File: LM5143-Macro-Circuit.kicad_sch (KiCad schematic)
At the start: 54 parts, among them J4 Conn_01x01_Socket, U1 LM5145, U2 NTMFS4D0N08XT1G, U3 NTMFS4D0N08XT1G, U4 NTMFS4D0N08XT1G, U5 NTMFS4D0N08XT1G

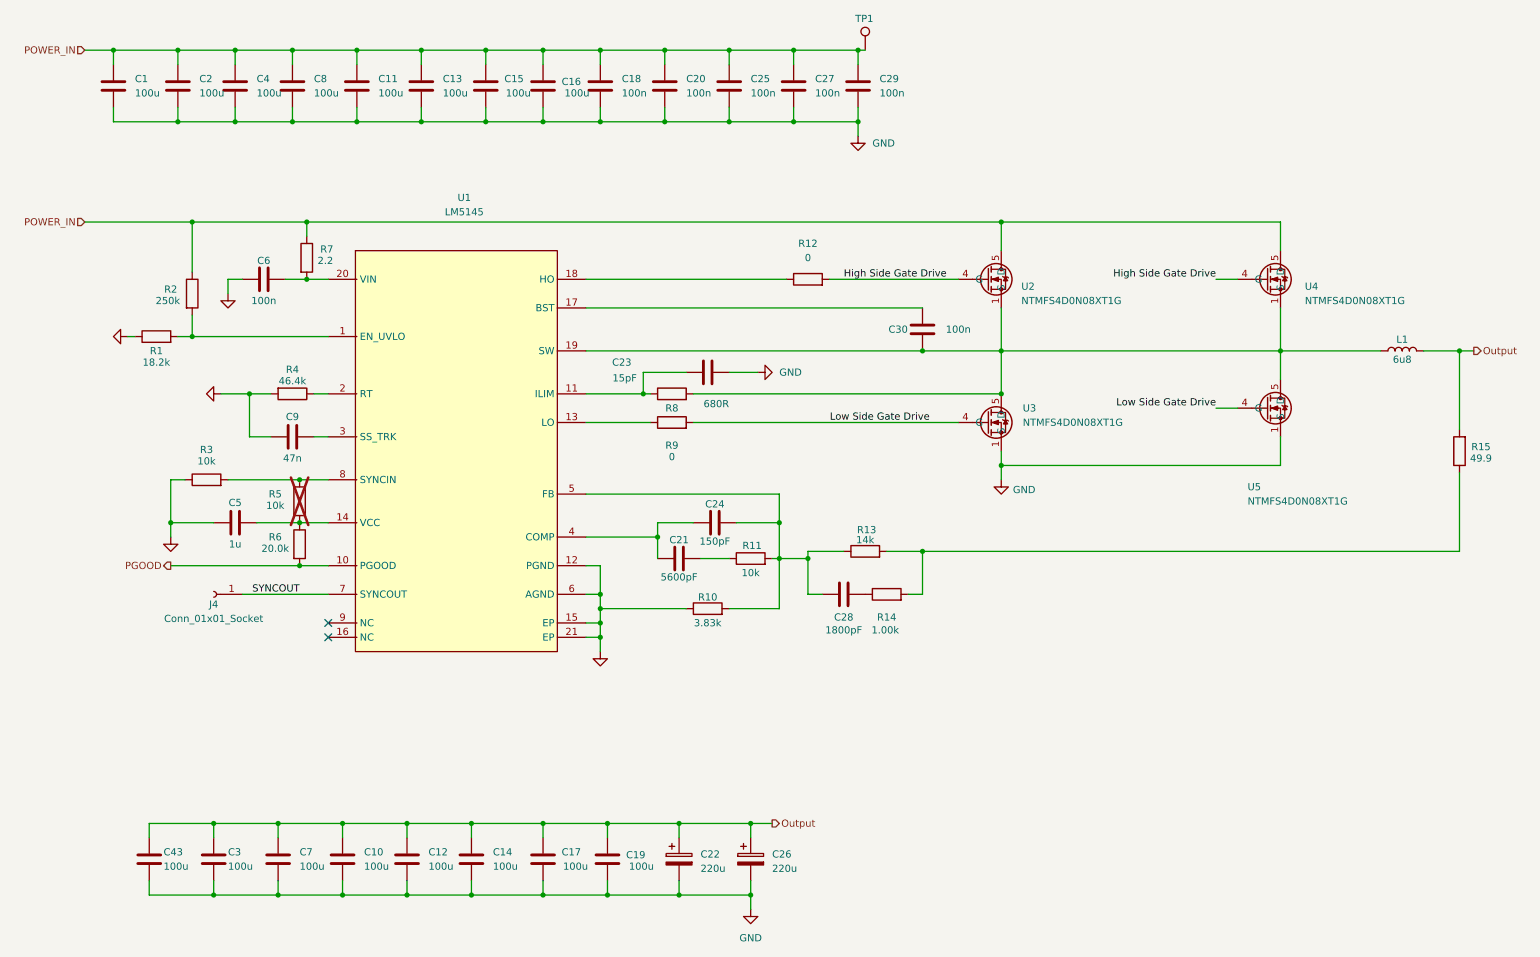
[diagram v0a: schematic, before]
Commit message: A
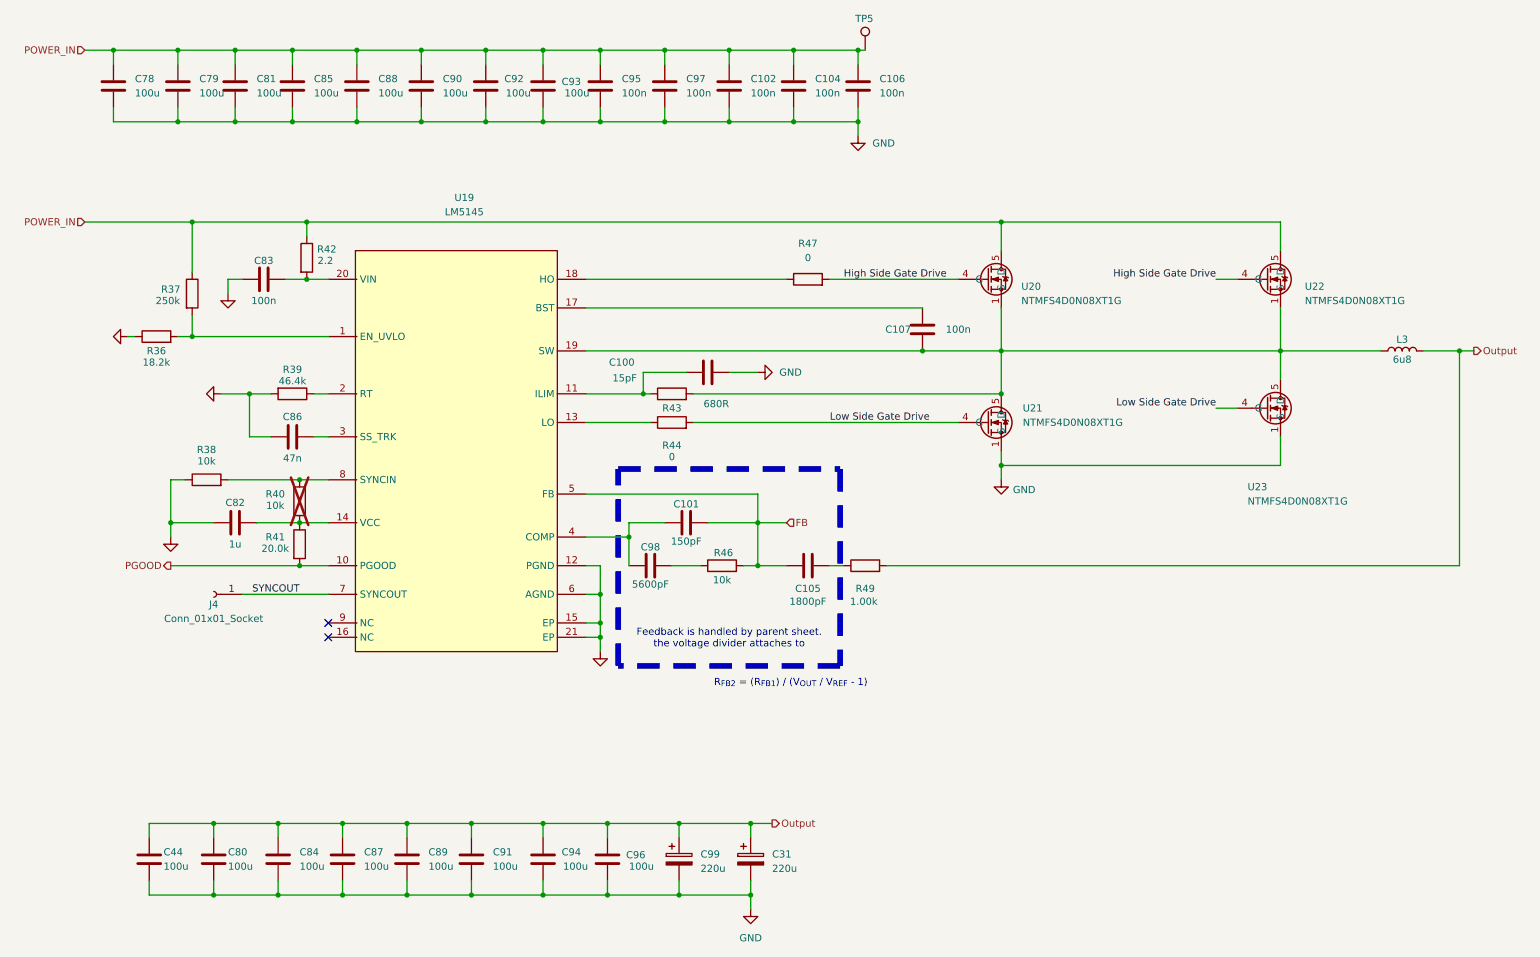
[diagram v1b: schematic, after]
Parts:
- removed R10: 3.83k, Resistor_SMD:R_0603_1608Metric, symbol Device:R
- removed R13: 14k, Resistor_SMD:R_0603_1608Metric, symbol Device:R
- removed R15: 49.9, Resistor_SMD:R_0603_1608Metric, symbol Device:R
- renumbered C23 to C100, C24 to C101, C25 to C102, C27 to C104, C28 to C105, C29 to C106, C30 to C107, C26 to C31, C43 to C44, C1 to C78, C2 to C79, C3 to C80, C4 to C81, C5 to C82, C6 to C83, C7 to C84, C8 to C85, C9 to C86, C10 to C87, C11 to C88, C12 to C89, C13 to C90, C14 to C91, C15 to C92, C16 to C93, C17 to C94, C18 to C95, C19 to C96, C20 to C97, C21 to C98, C22 to C99, L1 to L3, R1 to R36, R2 to R37, R3 to R38, R4 to R39, R5 to R40, R6 to R41, R7 to R42, R8 to R43, R9 to R44, R11 to R46, R12 to R47, R14 to R49, TP1 to TP5, U1 to U19, U2 to U20, U3 to U21, U4 to U22, U5 to U23
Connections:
- net Output: now also R49.2
- net FB: now reaches C101.2, C105.1, R46.2, U19.5 (FB)
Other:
- note added: "Feedback is handled by parent sheet. the voltage divider attaches to"
- note added: "R_{FB2} = (R_{FB1}) / (V_{OUT} / V_{REF} - 1)"
- moved on the sheet: C101, C105, C98, R46, R49
